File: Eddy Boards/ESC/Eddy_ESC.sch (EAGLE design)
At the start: 63 parts

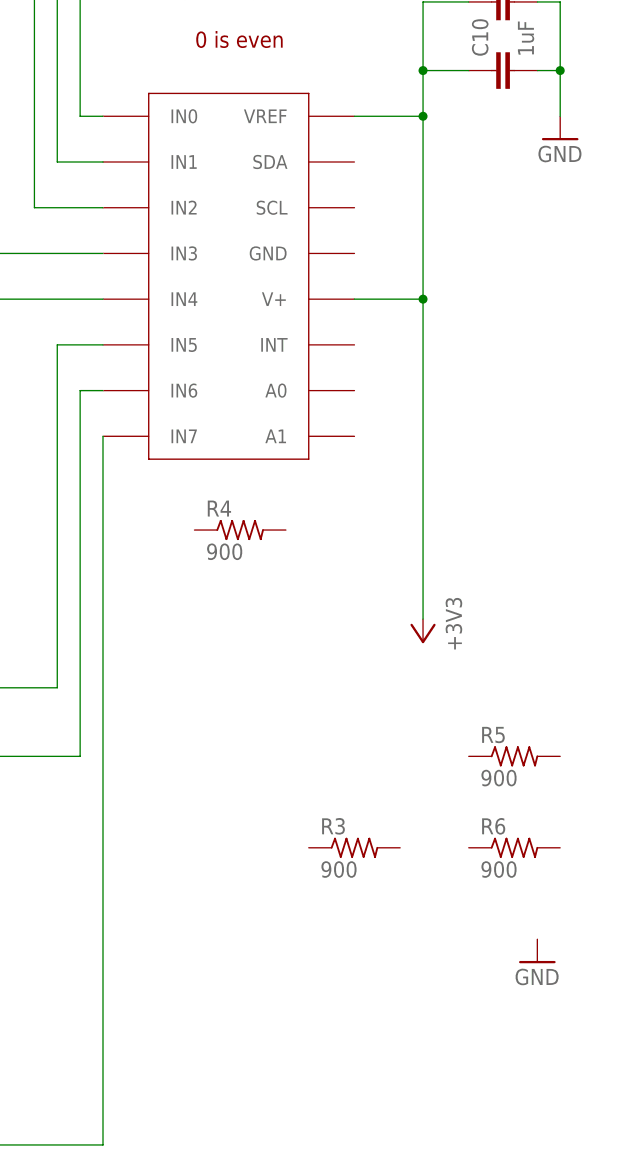
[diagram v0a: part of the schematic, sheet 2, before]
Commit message: temporary
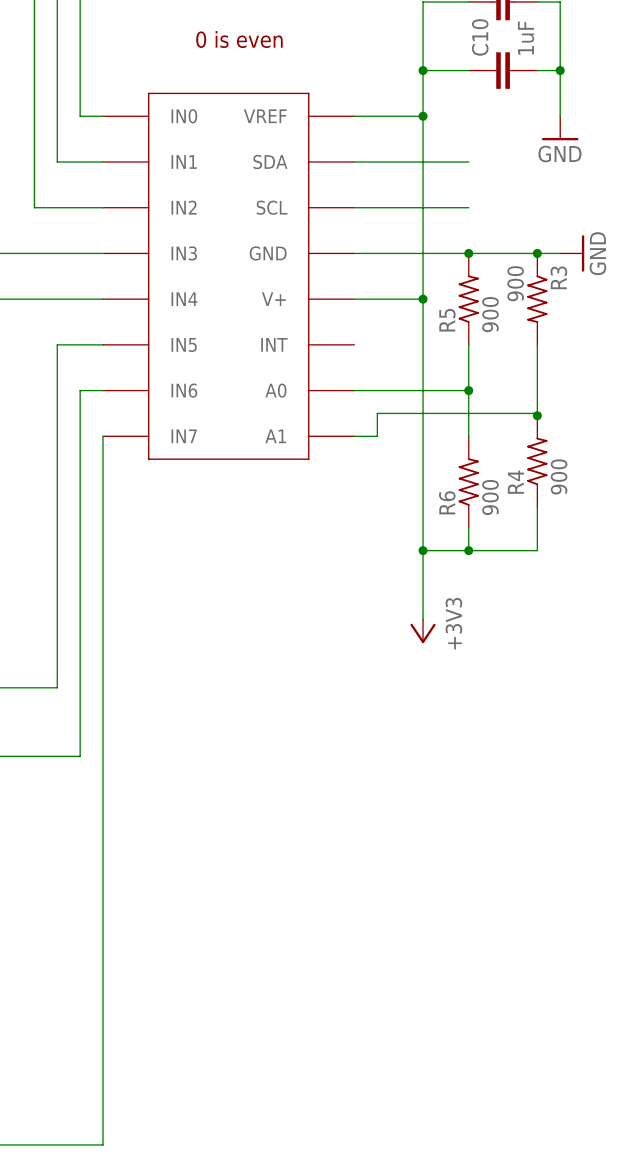
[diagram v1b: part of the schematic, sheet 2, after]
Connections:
- new net N$59: R5.1, R6.2, U$36.A0
- new net N$60: R3.2, R4.2, U$36.A1
- new net N$61: U$36.SDA
- new net N$62: U$36.SCL
- net +3V3: now also R4.1, R6.1
- net GND: now also R3.1, R5.2, U$36.GND
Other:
- moved on the sheet: R3, R4, R5, R6
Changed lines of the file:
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@@
 <attribute name="VALUE" x="167.64" y="50.8" size="1.778" layer="96"/>
 </instance>
-<instance part="GND7" gate="1" x="375.92" y="81.28" smashed="yes">
-<attribute name="VALUE" x="373.38" y="78.74" size="1.778" layer="96"/>
+<instance part="GND7" gate="1" x="381" y="160.02" smashed="yes" rot="R90">
+<attribute name="VALUE" x="383.54" y="157.48" size="1.778" layer="96" rot="R90"/>
 </instance>
 <instance part="U$28" gate="G$1" x="185.42" y="236.22" smashed="yes"/>
@@
 <attribute name="VALUE" x="365.76" y="121.92" size="1.778" layer="96" rot="R270"/>
 </instance>
-<instance part="R3" gate="G$1" x="355.6" y="93.98" smashed="yes">
-<attribute name="NAME" x="351.79" y="95.4786" size="1.778" layer="95"/>
-<attribute name="VALUE" x="351.79" y="90.678" size="1.778" layer="96"/>
-</instance>
-<instance part="R4" gate="G$1" x="342.9" y="129.286" smashed="yes">
-<attribute name="NAME" x="339.09" y="130.7846" size="1.778" layer="95"/>
-<attribute name="VALUE" x="339.09" y="125.984" size="1.778" layer="96"/>
-</instance>
-<instance part="R5" gate="G$1" x="373.38" y="104.14" smashed="yes">
-<attribute name="NAME" x="369.57" y="105.6386" size="1.778" layer="95"/>
-<attribute name="VALUE" x="369.57" y="100.838" size="1.778" layer="96"/>
-</instance>
-<instance part="R6" gate="G$1" x="373.38" y="93.98" smashed="yes">
-<attribute name="NAME" x="369.57" y="95.4786" size="1.778" layer="95"/>
-<attribute name="VALUE" x="369.57" y="90.678" size="1.778" layer="96"/>
+<instance part="R3" gate="G$1" x="375.92" y="154.94" smashed="yes" rot="R270">
+<attribute name="NAME" x="377.4186" y="158.75" size="1.778" layer="95" rot="R270"/>
+<attribute name="VALUE" x="372.618" y="158.75" size="1.778" layer="96" rot="R270"/>
+</instance>
+<instance part="R4" gate="G$1" x="375.92" y="136.906" smashed="yes" rot="R90">
+<attribute name="NAME" x="374.4214" y="133.096" size="1.778" layer="95" rot="R90"/>
+<attribute name="VALUE" x="379.222" y="133.096" size="1.778" layer="96" rot="R90"/>
+</instance>
+<instance part="R5" gate="G$1" x="368.3" y="154.94" smashed="yes" rot="R90">
+<attribute name="NAME" x="366.8014" y="151.13" size="1.778" layer="95" rot="R90"/>
+<attribute name="VALUE" x="371.602" y="151.13" size="1.778" layer="96" rot="R90"/>
+</instance>
+<instance part="R6" gate="G$1" x="368.3" y="134.62" smashed="yes" rot="R90">
+<attribute name="NAME" x="366.8014" y="130.81" size="1.778" layer="95" rot="R90"/>
+<attribute name="VALUE" x="371.602" y="130.81" size="1.778" layer="96" rot="R90"/>
 </instance>
 <instance part="C2" gate="G$1" x="149.86" y="246.38" smashed="yes" rot="R90">
@@
 <pinref part="GND4" gate="1" pin="GND"/>
 </segment>
+<segment>
+<pinref part="U$36" gate="G$1" pin="GND"/>
+<wire x1="355.6" y1="160.02" x2="368.3" y2="160.02" width="0.1524" layer="91"/>
+<pinref part="GND7" gate="1" pin="GND"/>
+<pinref part="R5" gate="G$1" pin="2"/>
+<wire x1="368.3" y1="160.02" x2="375.92" y2="160.02" width="0.1524" layer="91"/>
+<junction x="368.3" y="160.02"/>
+<pinref part="R3" gate="G$1" pin="1"/>
+<wire x1="375.92" y1="160.02" x2="378.46" y2="160.02" width="0.1524" layer="91"/>
+<junction x="375.92" y="160.02"/>
+</segment>
 </net>
 <net name="+3V3" class="0">
@@
 <segment>
 <pinref part="+3V2" gate="G$1" pin="+3V3"/>
-<wire x1="363.22" y1="119.38" x2="363.22" y2="154.94" width="0.1524" layer="91"/>
 <pinref part="C10" gate="G$1" pin="1"/>
+<wire x1="363.22" y1="119.38" x2="363.22" y2="127" width="0.1524" layer="91"/>
+<wire x1="363.22" y1="127" x2="363.22" y2="154.94" width="0.1524" layer="91"/>
 <wire x1="363.22" y1="154.94" x2="363.22" y2="175.26" width="0.1524" layer="91"/>
 <wire x1="363.22" y1="175.26" x2="363.22" y2="180.34" width="0.1524" layer="91"/>
@@
 <wire x1="355.6" y1="154.94" x2="363.22" y2="154.94" width="0.1524" layer="91"/>
 <junction x="363.22" y="154.94"/>
-</segment>
-</net>
+<wire x1="363.22" y1="127" x2="368.3" y2="127" width="0.1524" layer="91"/>
+<junction x="363.22" y="127"/>
+<pinref part="R4" gate="G$1" pin="1"/>
+<wire x1="368.3" y1="127" x2="375.92" y2="127" width="0.1524" layer="91"/>
+<wire x1="375.92" y1="127" x2="375.92" y2="131.826" width="0.1524" layer="91"/>
+<pinref part="R6" gate="G$1" pin="1"/>
+<wire x1="368.3" y1="129.54" x2="368.3" y2="127" width="0.1524" layer="91"/>
+<junction x="368.3" y="127"/>
+</segment>
+</net>
+<net name="N$59" class="0">
+<segment>
+<pinref part="U$36" gate="G$1" pin="A0"/>
+<wire x1="355.6" y1="144.78" x2="368.3" y2="144.78" width="0.1524" layer="91"/>
+<pinref part="R5" gate="G$1" pin="1"/>
+<wire x1="368.3" y1="144.78" x2="368.3" y2="149.86" width="0.1524" layer="91"/>
+<pinref part="R6" gate="G$1" pin="2"/>
+<wire x1="368.3" y1="144.78" x2="368.3" y2="139.7" width="0.1524" layer="91"/>
+<junction x="368.3" y="144.78"/>
+</segment>
+</net>
+<net name="N$60" class="0">
+<segment>
+<pinref part="U$36" gate="G$1" pin="A1"/>
+<wire x1="355.6" y1="139.7" x2="358.14" y2="139.7" width="0.1524" layer="91"/>
+<wire x1="358.14" y1="139.7" x2="358.14" y2="142.24" width="0.1524" layer="91"/>
+<pinref part="R4" gate="G$1" pin="2"/>
+<wire x1="358.14" y1="142.24" x2="375.92" y2="142.24" width="0.1524" layer="91"/>
+<wire x1="375.92" y1="142.24" x2="375.92" y2="141.986" width="0.1524" layer="91"/>
+<pinref part="R3" gate="G$1" pin="2"/>
+<wire x1="375.92" y1="141.986" x2="375.92" y2="149.86" width="0.1524" layer="91"/>
+<junction x="375.92" y="141.986"/>
+</segment>
+</net>
+<net name="N$61" class="0">
+<segment>
+<pinref part="U$36" gate="G$1" pin="SDA"/>
+<wire x1="355.6" y1="170.18" x2="368.3" y2="170.18" width="0.1524" layer="91"/>
+</segment>
+</net>
+<net name="N$62" class="0">
+<segment>
+<pinref part="U$36" gate="G$1" pin="SCL"/>
+<wire x1="355.6" y1="165.1" x2="368.3" y2="165.1" width="0.1524" layer="91"/>
+</segment>
+</net>
